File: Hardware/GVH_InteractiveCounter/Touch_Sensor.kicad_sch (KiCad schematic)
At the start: 9 parts, among them J4 Electrode, U1 AT42QT1010

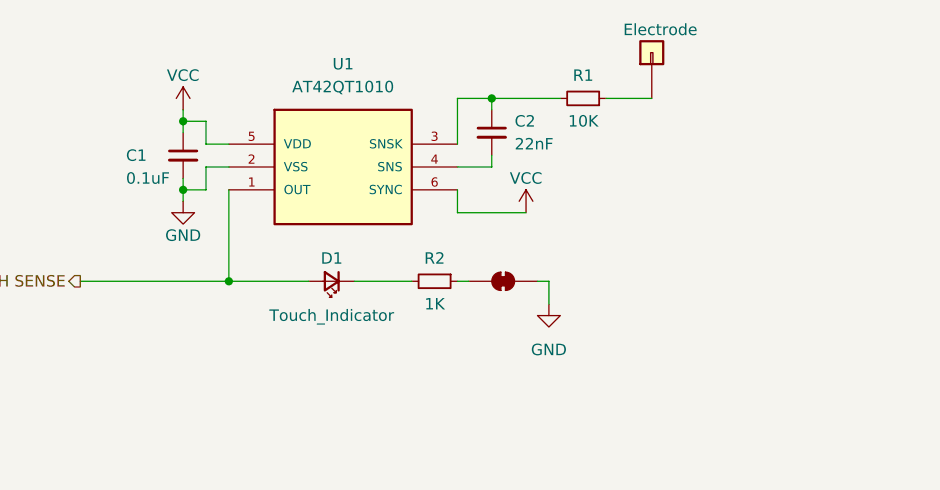
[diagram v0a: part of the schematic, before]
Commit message: Board version 2 done. Not happy will start over
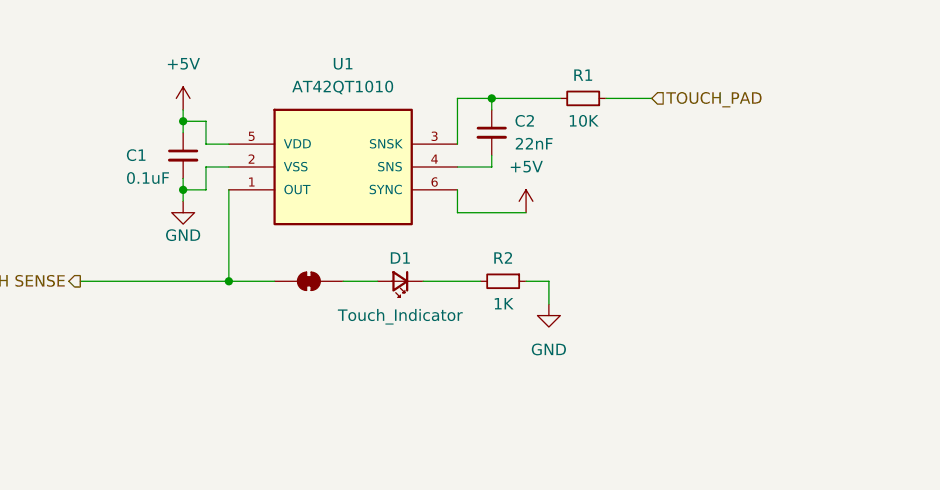
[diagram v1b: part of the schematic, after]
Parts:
- removed J4: Electrode, Connector_Pin:Pin_D1.3mm_L11.0mm_LooseFit, symbol Connector_Generic:Conn_01x01
- JP1: footprint Jumper:SolderJumper-2_P1.3mm_Bridged_RoundedPad1.0x1.5mm -> Jumper:SolderJumper-2_P1.3mm_Bridged_Pad1.0x1.5mm
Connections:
- net GND: now also R2.1; no longer JP1.2 (B)
- net TOUCH SENSE: now also JP1.1 (A); no longer D1.2 (A)
- net TOUCH_PAD: now reaches R1.1
- net VCC renamed +5V
- new net: D1.2 (A), JP1.2 (B)
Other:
- moved on the sheet: D1, R2
